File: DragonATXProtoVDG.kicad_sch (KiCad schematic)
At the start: 73 parts, among them IC1 74LS273, IC2 MC6847, IC3 MC14053, J3 JTAG, Q1 MMBT4401, Q2 NPN, Q3 NPN, Q4 NPN, Q5 NPN, Q6 NPN, U1 AD724JR, U2 74LS244, U3 ATF1502ASL-xAx44, U4 74LS244, U5 74LS244, Y2 4.433618MHz

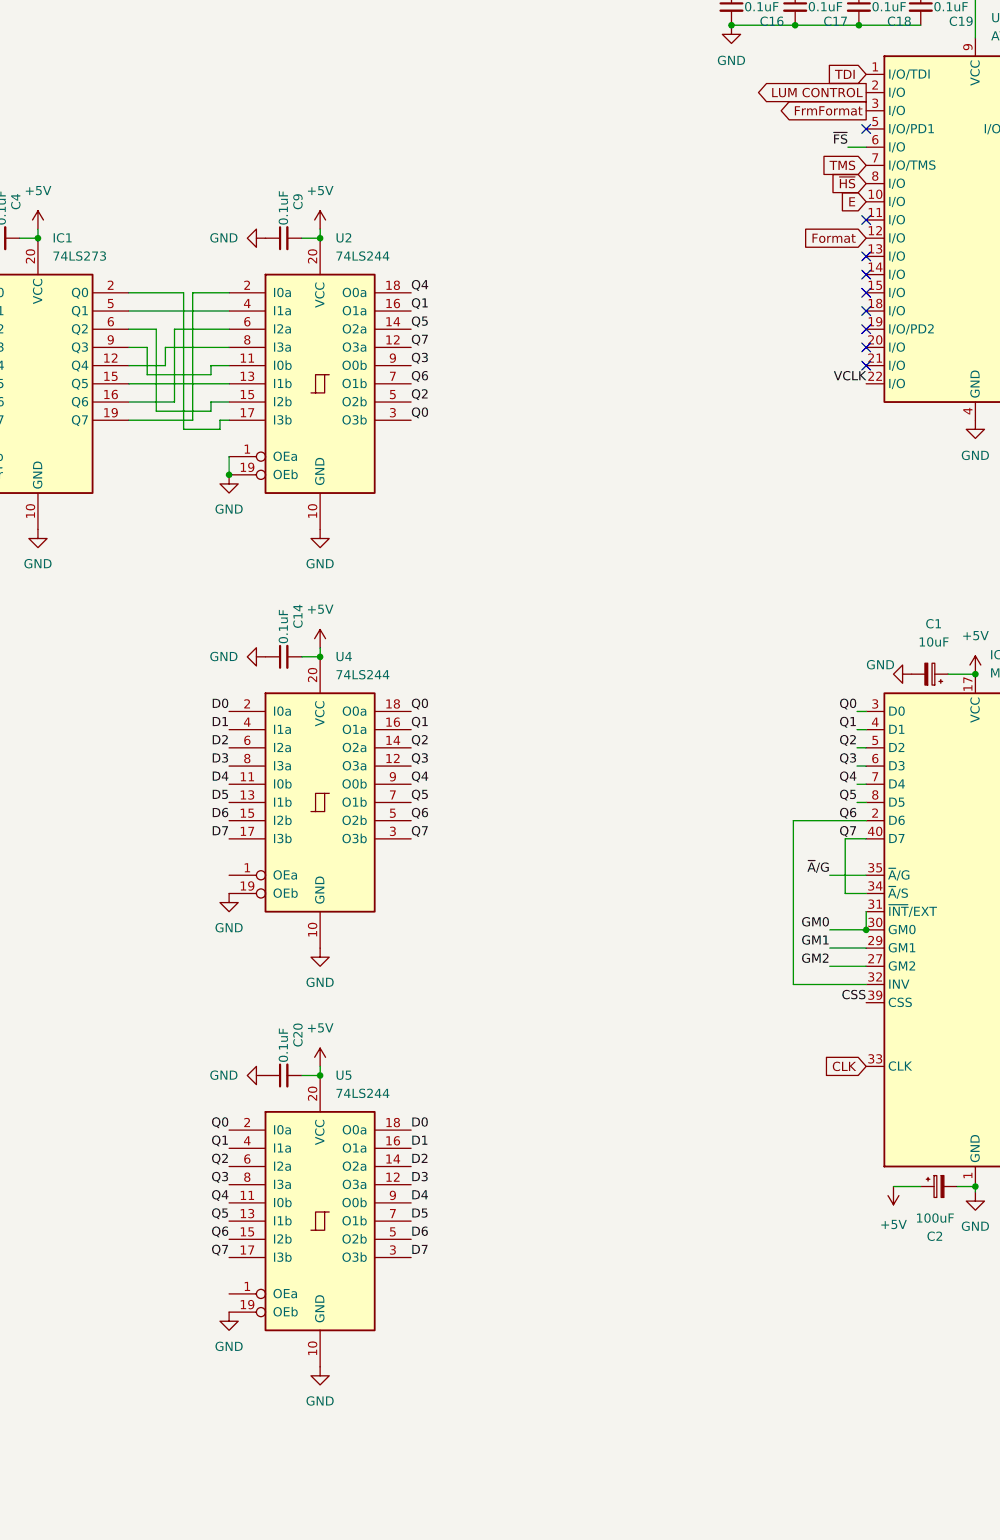
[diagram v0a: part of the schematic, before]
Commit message: update
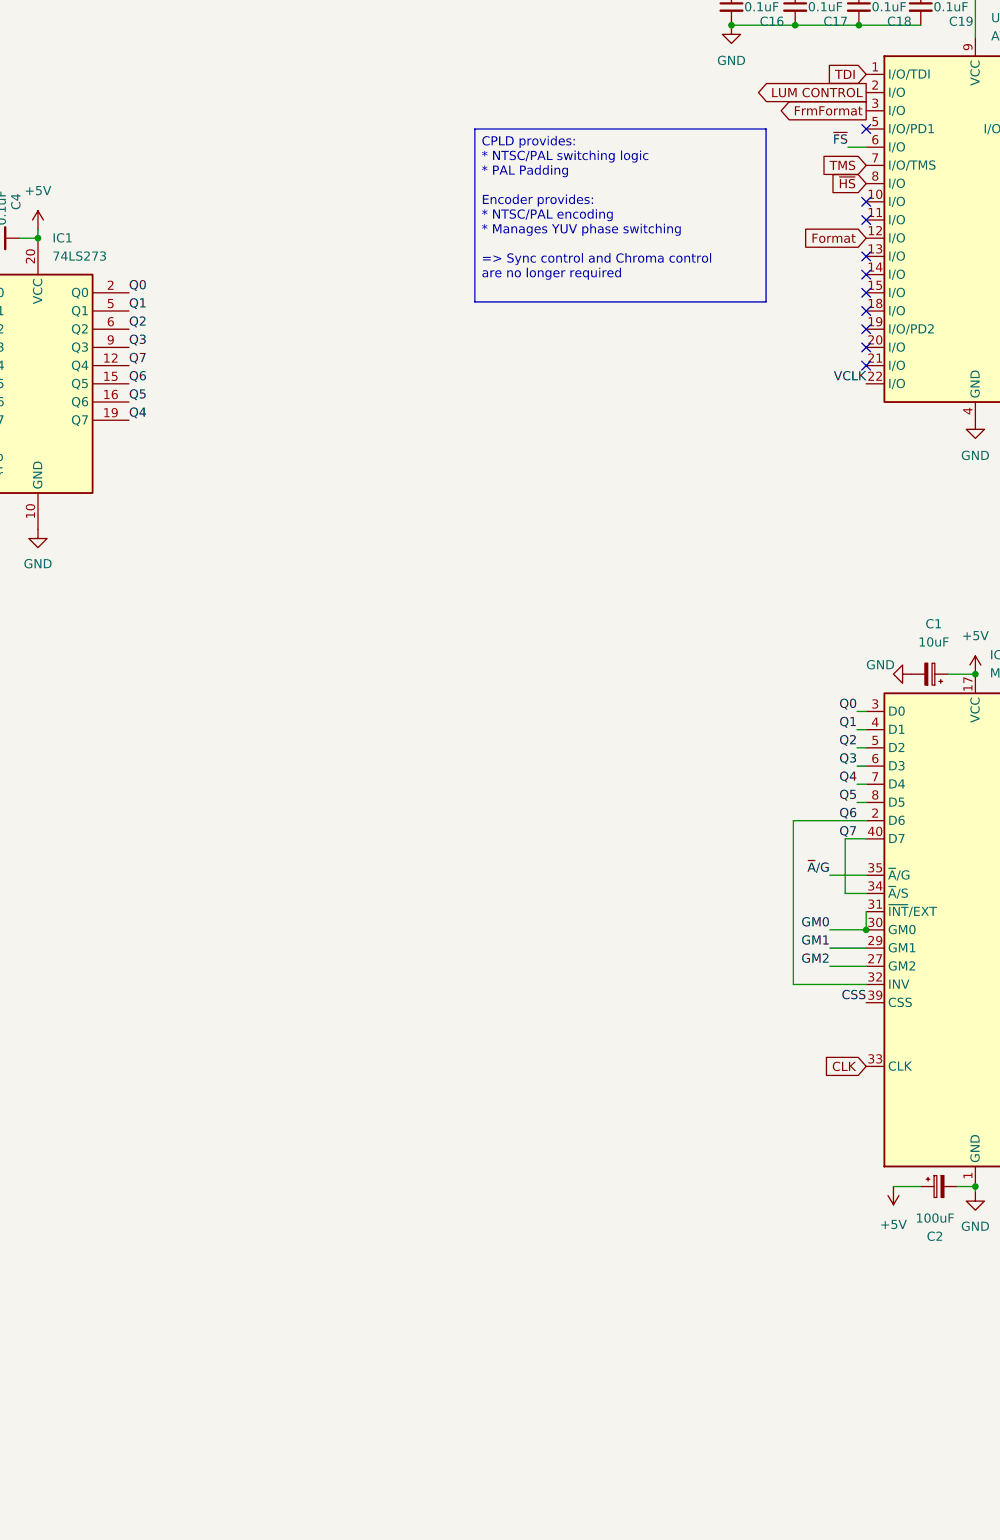
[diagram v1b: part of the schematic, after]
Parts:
- removed C14, C20, C9: 0.1uF, Capacitor_SMD:C_0805_2012Metric_Pad1.18x1.45mm_HandSolder, symbol Device:C_Small
- removed U2, U4, U5: 74LS244, PCM_Package_SO_AKL:SO-20_5.3x12.6mm_P1.27mm, symbol 74xx:74LS244
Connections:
- net E: no longer U3.10 (I/O)
- net Q0: now also IC1.2 (Q0)
- net Q1: now also IC1.5 (Q1)
- net Q2: now also IC1.6 (Q2)
- net Q3: now also IC1.9 (Q3)
- net Q4: now also IC1.19 (Q7)
- net Q5: now also IC1.16 (Q6)
- net Q6: now also IC1.15 (Q5)
- net Q7: now also IC1.12 (Q4)
- no-connect marks 55 -> 56
